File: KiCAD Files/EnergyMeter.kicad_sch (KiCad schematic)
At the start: 7 parts, among them J1 Screw_Terminal_AC

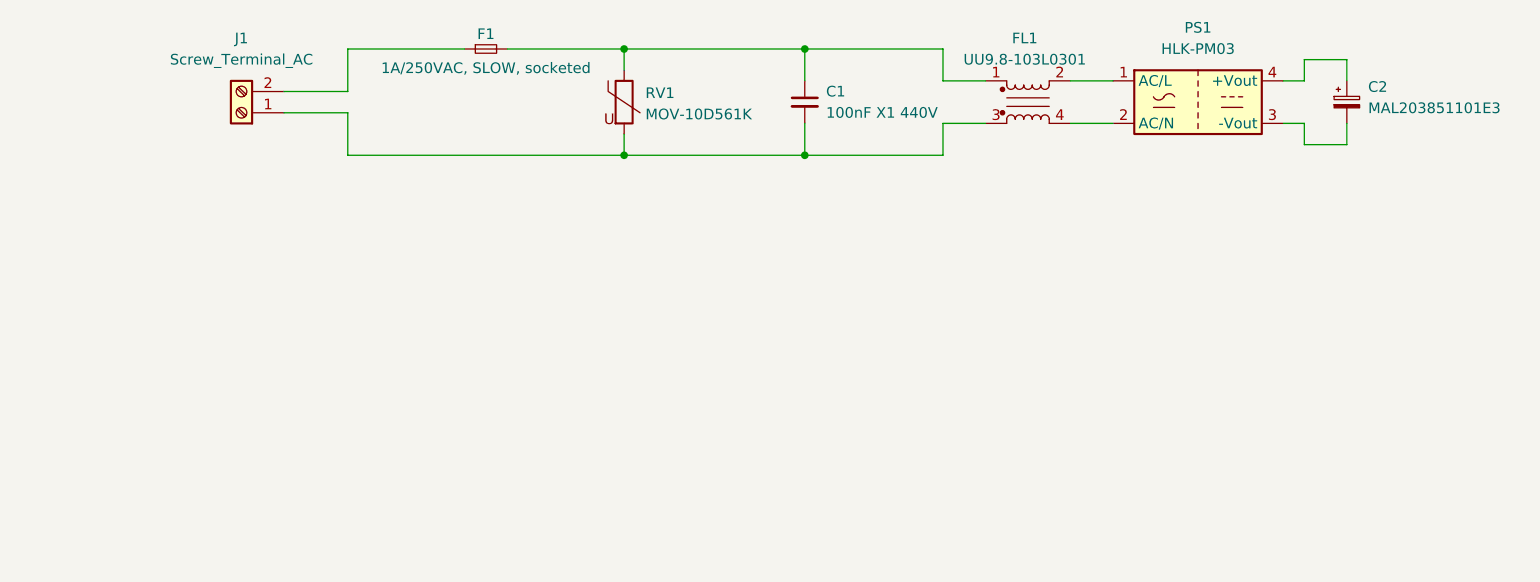
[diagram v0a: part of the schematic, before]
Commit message: update
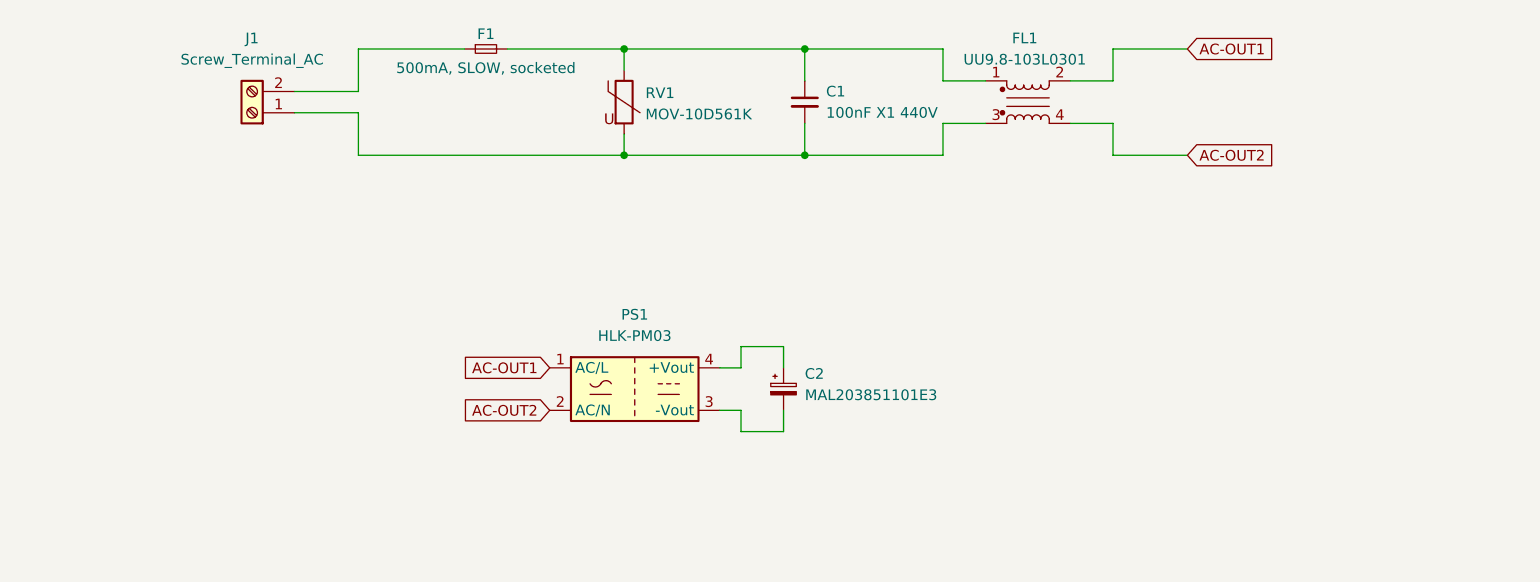
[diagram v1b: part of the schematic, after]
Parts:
- F1: value 1A/250VAC, SLOW, socketed -> 500mA, SLOW, socketed
- J1: LCSC Part # C409161 -> C707824
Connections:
- net AC-OUT1: now reaches FL1.2, PS1.1 (AC/L)
- net AC-OUT2: now reaches FL1.4, PS1.2 (AC/N)
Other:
- moved on the sheet: C2, J1, PS1
